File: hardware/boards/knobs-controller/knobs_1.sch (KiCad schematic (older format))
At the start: 28 parts, among them J1 ZX62-AB-5PA(31), J4 JST---S4B-PH-SM4-TB(LF)(SN)_J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, J8 2X3_SMD_MALE, U3 ATSAMD21G18A-48, Y1 32.768KHz

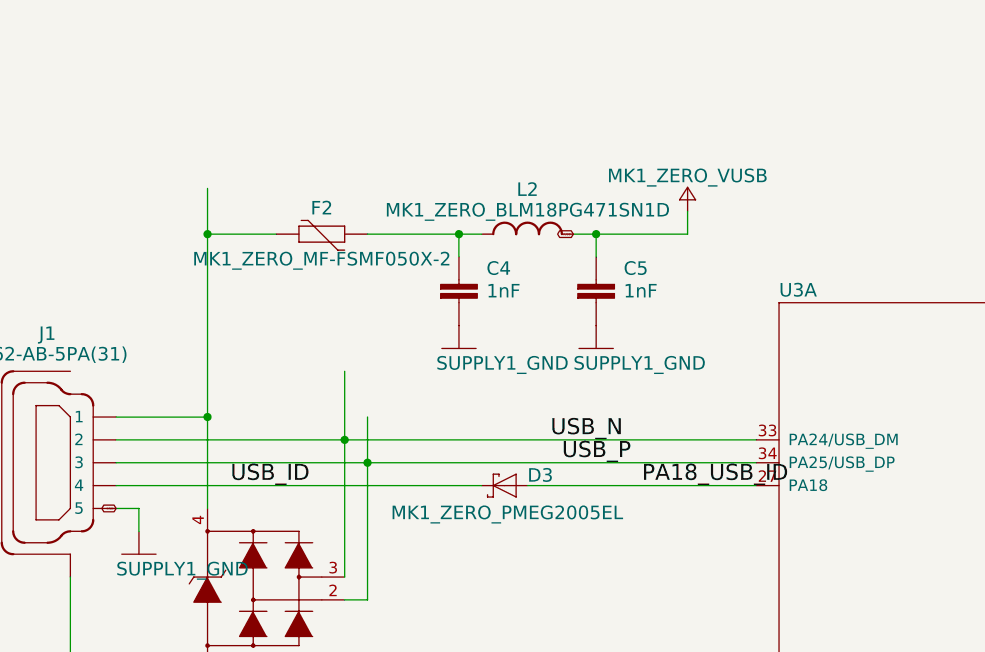
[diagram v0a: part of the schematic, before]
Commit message: minor cleanup
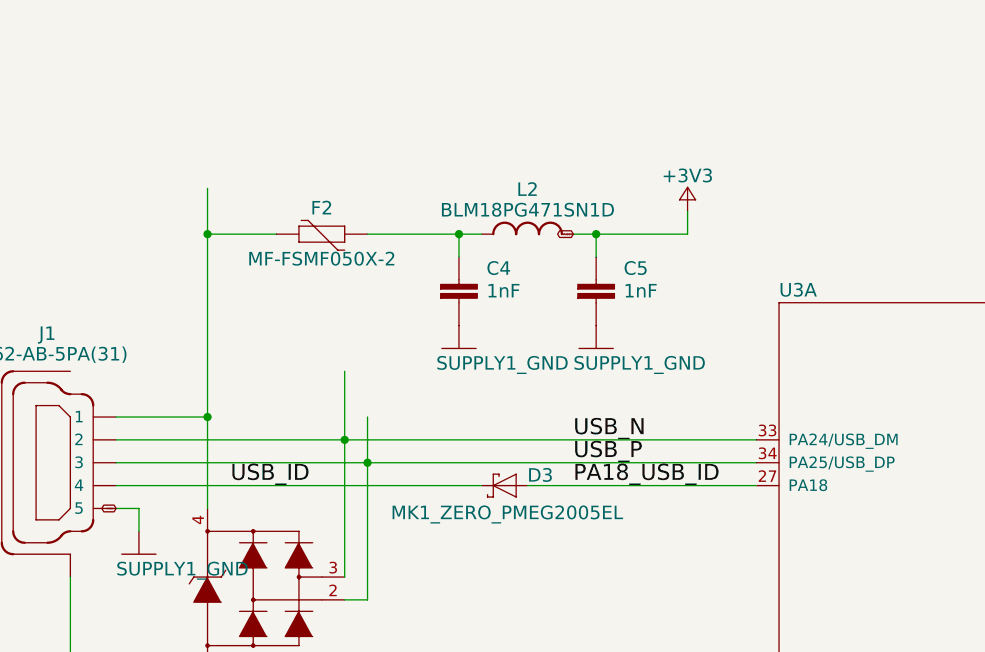
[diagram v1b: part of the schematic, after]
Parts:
- F2: value MK1_ZERO_MF-FSMF050X-2 -> MF-FSMF050X-2
- L2: value MK1_ZERO_BLM18PG471SN1D -> BLM18PG471SN1D
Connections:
- net labels removed: MK1_ZERO_VUSB
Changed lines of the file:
@@
 Wire Wire Line
 	3400 3400 4400 3400
-Text Label 3900 3400 0    70   ~ 0
+Text Label 3600 3400 0    70   ~ 0
 PA18_USB_ID
 Wire Wire Line
@@
 	2700 3100 2700 3300
 Connection ~ 2700 3300
-Text Label 3550 3300 0    70   ~ 0
+Text Label 3600 3300 0    70   ~ 0
 USB_P
 Wire Wire Line
@@
 	2600 2900 2600 3200
 Connection ~ 2600 3200
-Text Label 3500 3200 0    70   ~ 0
+Text Label 3600 3200 0    70   ~ 0
 USB_N
 Wire Wire Line
@@
 $EndComp
 $Comp
-L knobs-eagle-import:MK1_ZERO_BLM18PG471SN1D L2
-U 1 1 9F8286A9
-P 3400 2300
-AR Path="/9F8286A9" Ref="L2"  Part="1"
-AR Path="/5D86641C/9F8286A9" Ref="L2"  Part="1"
-F 0 "L2" H 3400 2460 59  0000 C BNN
-F 1 "MK1_ZERO_BLM18PG471SN1D" H 3400 2370 59  0000 C BNN
-F 2 "knobs:MK1_ZERO_0603-1608X90N" H 3400 2300 50  0001 C CNN
-F 3 "" H 3400 2300 50  0001 C CNN
-	1    3400 2300
-	1    0    0    -1
-$EndComp
-$Comp
 L knobs-eagle-import:MK1_ZERO_PRTR5V0U2X,215 D1
 U 1 1 DA5D11AB
@@
 $EndComp
 $Comp
-L knobs-eagle-import:MK1_ZERO_VUSB #U$2
-U 1 1 6197D135
-P 4100 2100
-AR Path="/6197D135" Ref="#U$2"  Part="1"
-AR Path="/5D86641C/6197D135" Ref="#U$02"  Part="1"
-F 0 "#U$02" H 4100 2100 50  0001 C CNN
-F 1 "MK1_ZERO_VUSB" H 4100 2120 59  0000 C BNN
-F 2 "" H 4100 2100 50  0001 C CNN
-F 3 "" H 4100 2100 50  0001 C CNN
-	1    4100 2100
-	1    0    0    -1
-$EndComp
-$Comp
 L knobs-eagle-import:SUPPLY1_GND #GND9
 U 1 1 158B4DC7
@@
 AR Path="/5D86641C/5B319BB3" Ref="F2"  Part="1"
 F 0 "F2" V 2579 2300 59  0000 C TNN
-F 1 "MK1_ZERO_MF-FSMF050X-2" V 2425 2300 59  0000 C BNN
+F 1 "MF-FSMF050X-2" V 2425 2300 59  0000 C BNN
 F 2 "knobs:MK1_ZERO_0603-F1608X100N" H 2500 2300 50  0001 C CNN
 F 3 "" H 2500 2300 50  0001 C CNN
@@
 Wire Bus Line
 	7800 7200 7800 9600
+$Comp
+L knobs-eagle-import:MK1_ZERO_BLM18PG471SN1D L2
+U 1 1 9F8286A9
+P 3400 2300
+AR Path="/9F8286A9" Ref="L2"  Part="1"
+AR Path="/5D86641C/9F8286A9" Ref="L2"  Part="1"
+F 0 "L2" H 3400 2460 59  0000 C BNN
+F 1 "BLM18PG471SN1D" H 3400 2370 59  0000 C BNN
+F 2 "knobs:MK1_ZERO_0603-1608X90N" H 3400 2300 50  0001 C CNN
+F 3 "" H 3400 2300 50  0001 C CNN
+	1    3400 2300
+	1    0    0    -1
+$EndComp
+$Comp
+L knobs-eagle-import:+3V3 #+3V?
+U 1 1 5D890552
+P 4100 2100
+AR Path="/5D890552" Ref="#+3V?"  Part="1"
+AR Path="/5D86641C/5D890552" Ref="#+3V?"  Part="1"
+F 0 "#+3V?" H 4100 2100 50  0001 C CNN
+F 1 "+3V3" H 4100 2120 59  0000 C BNN
+F 2 "" H 4100 2100 50  0001 C CNN
+F 3 "" H 4100 2100 50  0001 C CNN
+	1    4100 2100
+	1    0    0    -1
+$EndComp
 $EndSCHEMATC
